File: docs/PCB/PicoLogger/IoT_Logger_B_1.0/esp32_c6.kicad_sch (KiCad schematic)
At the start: 23 parts, among them J2 ESP_UART, Q1 BSS138, Q2 AO3407, SW1 Tact Switch 6x6mm / 13mm, SW2 Tact Switch 6x6mm / 13mm, U2 ESP32-C6-WROOM-1U

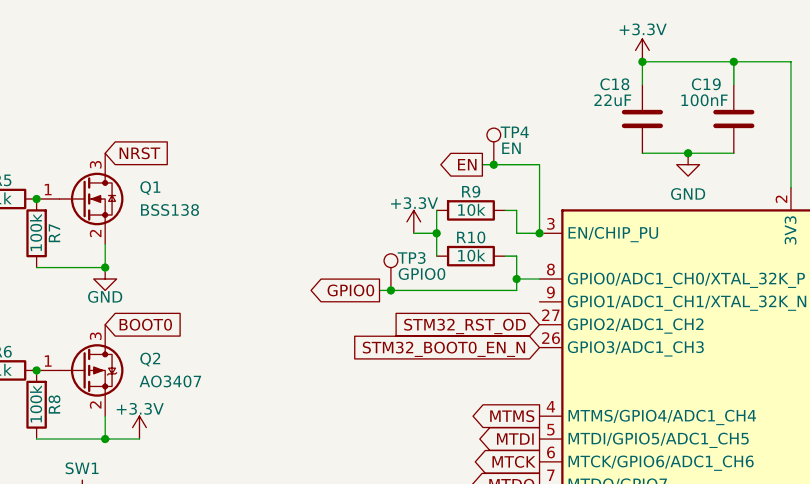
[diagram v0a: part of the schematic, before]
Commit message: Code added, documentation review.
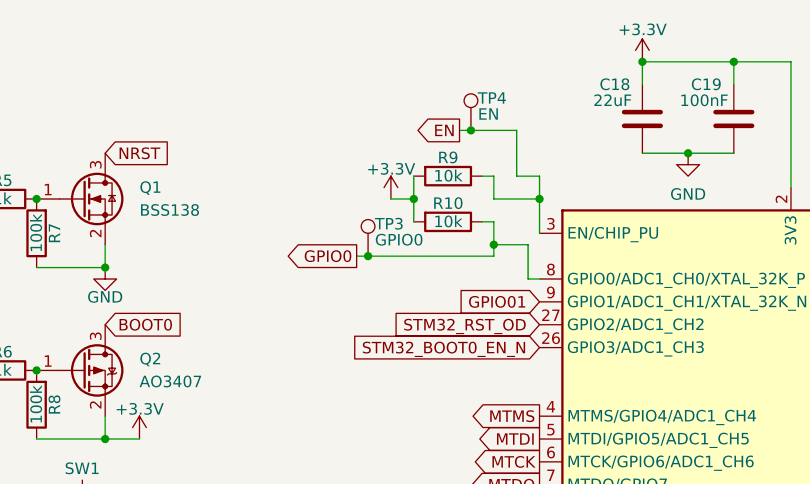
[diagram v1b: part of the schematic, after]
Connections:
- net GPIO01: now reaches U2.9 (GPIO1/ADC1_CH1/XTAL_32K_N)
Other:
- moved on the sheet: R10, R9, TP3, TP4
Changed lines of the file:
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@@
 	)
 	(junction
-		(at 111.76 80.01)
+		(at 109.22 76.2)
 		(diameter 0)
 		(color 0 0 0 0)
@@
 	)
 	(junction
-		(at 123.19 66.04)
+		(at 120.65 62.23)
 		(diameter 0)
 		(color 0 0 0 0)
@@
 	)
 	(junction
-		(at 125.73 78.74)
+		(at 123.19 74.93)
 		(diameter 0)
 		(color 0 0 0 0)
 	)
 	(junction
-		(at 116.84 73.66)
+		(at 128.27 69.85)
 		(diameter 0)
 		(color 0 0 0 0)
 	)
 	(junction
-		(at 72.39 88.9)
+		(at 114.3 69.85)
 		(diameter 0)
 		(color 0 0 0 0)
 	)
 	(junction
-		(at 149.86 54.61)
+		(at 72.39 88.9)
 		(diameter 0)
 		(color 0 0 0 0)
 	)
 	(junction
-		(at 128.27 73.66)
+		(at 149.86 54.61)
 		(diameter 0)
 		(color 0 0 0 0)
@@
 	(wire
 		(pts
-			(xy 125.73 71.12) (xy 125.73 73.66)
+			(xy 123.19 67.31) (xy 123.19 69.85)
+		)
+		(stroke
+			(width 0)
+			(type default)
+		)
+	)
+	(wire
+		(pts
+			(xy 128.27 67.31) (xy 128.27 69.85)
 		)
 		(stroke
@@
 	(wire
 		(pts
-			(xy 125.73 80.01) (xy 125.73 78.74)
+			(xy 123.19 76.2) (xy 123.19 74.93)
 		)
 		(stroke
@@
 	(wire
 		(pts
-			(xy 125.73 73.66) (xy 128.27 73.66)
+			(xy 123.19 69.85) (xy 128.27 69.85)
 		)
 		(stroke
@@
 	(wire
 		(pts
+			(xy 127 74.93) (xy 127 78.74)
+		)
+		(stroke
+			(width 0)
+			(type default)
+		)
+	)
+	(wire
+		(pts
 			(xy 193.04 69.85) (xy 193.04 73.66)
 		)
@@
 	(wire
 		(pts
-			(xy 116.84 73.66) (xy 116.84 76.2)
+			(xy 127 78.74) (xy 128.27 78.74)
 		)
 		(stroke
@@
 	(wire
 		(pts
-			(xy 128.27 66.04) (xy 128.27 73.66)
+			(xy 114.3 69.85) (xy 114.3 72.39)
+		)
+		(stroke
+			(width 0)
+			(type default)
+		)
+	)
+	(wire
+		(pts
+			(xy 125.73 62.23) (xy 125.73 67.31)
 		)
 		(stroke
@@
 	(wire
 		(pts
-			(xy 114.3 73.66) (xy 116.84 73.66)
+			(xy 111.76 69.85) (xy 114.3 69.85)
 		)
 		(stroke
@@
 	(wire
 		(pts
-			(xy 111.76 80.01) (xy 125.73 80.01)
+			(xy 109.22 76.2) (xy 123.19 76.2)
 		)
 		(stroke
@@
 	(wire
 		(pts
-			(xy 116.84 71.12) (xy 116.84 73.66)
+			(xy 114.3 67.31) (xy 114.3 69.85)
 		)
 		(stroke
@@
 	(wire
 		(pts
-			(xy 121.92 66.04) (xy 123.19 66.04)
+			(xy 119.38 62.23) (xy 120.65 62.23)
 		)
 		(stroke
@@
 	(wire
 		(pts
-			(xy 125.73 78.74) (xy 128.27 78.74)
+			(xy 123.19 74.93) (xy 127 74.93)
 		)
 		(stroke
@@
 	(wire
 		(pts
-			(xy 124.46 76.2) (xy 125.73 76.2)
+			(xy 121.92 72.39) (xy 123.19 72.39)
 		)
 		(stroke
@@
 	(wire
 		(pts
-			(xy 124.46 71.12) (xy 125.73 71.12)
+			(xy 121.92 67.31) (xy 123.19 67.31)
+		)
+		(stroke
+			(width 0)
+			(type default)
+		)
+	)
+	(wire
+		(pts
+			(xy 125.73 67.31) (xy 128.27 67.31)
+		)
+		(stroke
+			(width 0)
+			(type default)
+		)
+	)
+	(wire
+		(pts
+			(xy 123.19 72.39) (xy 123.19 74.93)
 		)
 		(stroke
@@
 	(wire
 		(pts
-			(xy 125.73 76.2) (xy 125.73 78.74)
+			(xy 120.65 62.23) (xy 125.73 62.23)
 		)
 		(stroke
@@
 	(wire
 		(pts
-			(xy 123.19 66.04) (xy 128.27 66.04)
+			(xy 128.27 69.85) (xy 128.27 73.66)
 		)
 		(stroke
@@
 	(wire
 		(pts
-			(xy 110.49 80.01) (xy 111.76 80.01)
+			(xy 107.95 76.2) (xy 109.22 76.2)
 		)
 		(stroke
@@
 	(global_label "EN"
 		(shape output)
-		(at 121.92 66.04 180)
+		(at 119.38 62.23 180)
 		(fields_autoplaced yes)
 		(effects
@@
 		)
 		(property "Intersheetrefs" "${INTERSHEET_REFS}"
-			(at 116.4553 66.04 0)
+			(at 113.9153 62.23 0)
 			(effects
 				(font
@@
 	(global_label "GPIO0"
 		(shape output)
-		(at 110.49 80.01 180)
+		(at 107.95 76.2 180)
 		(fields_autoplaced yes)
 		(effects
@@
 		)
 		(property "Intersheetrefs" "${INTERSHEET_REFS}"
-			(at 101.82 80.01 0)
+			(at 99.28 76.2 0)
 			(effects
 				(font
@@
 		)
 	)
+	(global_label "GPIO01"
+		(shape input)
+		(at 128.27 81.28 180)
+		(fields_autoplaced yes)
+		(effects
+			(font
+				(size 1.27 1.27)
+			)
+			(justify right)
+		)
+		(property "Intersheetrefs" "${INTERSHEET_REFS}"
+			(at 118.3905 81.28 0)
+			(effects
+				(font
+					(size 1.27 1.27)
+				)
+				(justify right)
+				(hide yes)
+			)
+		)
+	)
 	(global_label "USART2_RX"
 		(shape input)
@@
 	(symbol
 		(lib_id "power:+3.3V")
-		(at 114.3 73.66 0)
+		(at 111.76 69.85 0)
 		(unit 1)
 		(exclude_from_sim no)
@@
 		(dnp no)
 		(property "Reference" "#PWR031"
-			(at 114.3 77.47 0)
+			(at 111.76 73.66 0)
 			(effects
 				(font
@@
 		)
 		(property "Value" "+3.3V"
-			(at 114.3 70.358 0)
+			(at 111.76 66.548 0)
 			(effects
 				(font
@@
 		)
 		(property "Footprint" ""
-			(at 114.3 73.66 0)
+			(at 111.76 69.85 0)
 			(effects
 				(font
@@
 		)
 		(property "Datasheet" ""
-			(at 114.3 73.66 0)
+			(at 111.76 69.85 0)
 			(effects
 				(font
@@
 		)
 		(property "Description" "Power symbol creates a global label with name \"+3.3V\""
-			(at 114.3 73.66 0)
+			(at 111.76 69.85 0)
 			(effects
 				(font
@@
 	(symbol
 		(lib_id "Device:R")
-		(at 120.65 71.12 270)
+		(at 118.11 67.31 270)
 		(unit 1)
 		(exclude_from_sim no)
@@
 		(dnp no)
 		(property "Reference" "R9"
-			(at 120.65 69.088 90)
+			(at 118.11 65.278 90)
 			(effects
 				(font
@@
 		)
 		(property "Value" "10k"
-			(at 120.65 71.12 90)
+			(at 118.11 67.31 90)
 			(effects
 				(font
@@
 		)
 		(property "Footprint" "Resistor_SMD:R_0603_1608Metric"
-			(at 120.65 69.342 90)
+			(at 118.11 65.532 90)
 			(effects
 				(font
@@
 		)
 		(property "Datasheet" "~"
-			(at 120.65 71.12 0)
+			(at 118.11 67.31 0)
 			(effects
 				(font
@@
 		)
 		(property "Description" "Resistor"
-			(at 120.65 71.12 0)
+			(at 118.11 67.31 0)
 			(effects
 				(font
@@
 		)
 		(property "Sim.Library" ""
-			(at 120.65 71.12 90)
+			(at 118.11 67.31 90)
 			(effects
 				(font
@@
 	(symbol
 		(lib_id "Connector:TestPoint")
-		(at 111.76 80.01 0)
+		(at 109.22 76.2 0)
 		(unit 1)
 		(exclude_from_sim no)
@@
 		(dnp no)
 		(property "Reference" "TP3"
-			(at 112.522 76.454 0)
+			(at 109.982 72.644 0)
 			(effects
 				(font
@@
 		)
 		(property "Value" "GPIO0"
-			(at 112.522 78.232 0)
+			(at 109.982 74.422 0)
 			(effects
 				(font
@@
 		)
 		(property "Footprint" "TestPoint:TestPoint_Pad_D1.5mm"
-			(at 116.84 80.01 0)
+			(at 114.3 76.2 0)
 			(effects
 				(font
@@
 		)
 		(property "Datasheet" "~"
-			(at 116.84 80.01 0)
+			(at 114.3 76.2 0)
 			(effects
 				(font
@@
 		)
 		(property "Description" "test point"
-			(at 111.76 80.01 0)
+			(at 109.22 76.2 0)
 			(effects
 				(font
@@
 	(symbol
 		(lib_id "Device:R")
-		(at 120.65 76.2 270)
+		(at 118.11 72.39 270)
 		(unit 1)
 		(exclude_from_sim no)
@@
 		(dnp no)
 		(property "Reference" "R10"
-			(at 120.65 74.168 90)
+			(at 118.11 70.358 90)
 			(effects
 				(font
@@
 		)
 		(property "Value" "10k"
-			(at 120.65 76.2 90)
+			(at 118.11 72.39 90)
 			(effects
 				(font
@@
 		)
 		(property "Footprint" "Resistor_SMD:R_0603_1608Metric"
-			(at 120.65 74.422 90)
+			(at 118.11 70.612 90)
 			(effects
 				(font
@@
 		)
 		(property "Datasheet" "~"
-			(at 120.65 76.2 0)
+			(at 118.11 72.39 0)
 			(effects
 				(font
@@
 		)
 		(property "Description" "Resistor"
-			(at 120.65 76.2 0)
+			(at 118.11 72.39 0)
 			(effects
 				(font
@@
 		)
 		(property "Sim.Library" ""
-			(at 120.65 76.2 90)
+			(at 118.11 72.39 90)
 			(effects
 				(font
@@
 	(symbol
 		(lib_id "Connector:TestPoint")
-		(at 123.19 66.04 0)
+		(at 120.65 62.23 0)
 		(unit 1)
 		(exclude_from_sim no)
@@
 		(dnp no)
 		(property "Reference" "TP4"
-			(at 123.952 62.484 0)
+			(at 121.412 58.674 0)
 			(effects
 				(font
@@
 		)
 		(property "Value" "EN"
-			(at 123.952 64.262 0)
+			(at 121.412 60.452 0)
 			(effects
 				(font
@@
 		)
 		(property "Footprint" "TestPoint:TestPoint_Pad_D1.5mm"
-			(at 128.27 66.04 0)
+			(at 125.73 62.23 0)
 			(effects
 				(font
@@
 		)
 		(property "Datasheet" "~"
-			(at 128.27 66.04 0)
+			(at 125.73 62.23 0)
 			(effects
 				(font
@@
 		)
 		(property "Description" "test point"
-			(at 123.19 66.04 0)
+			(at 120.65 62.23 0)
 			(effects
 				(font
